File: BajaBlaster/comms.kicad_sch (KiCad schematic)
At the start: 6 parts, among them J2 Conn_01x06_Pin, J3 INTERBOARD, J4 Conn_01x04_Pin, U4 TCAN330

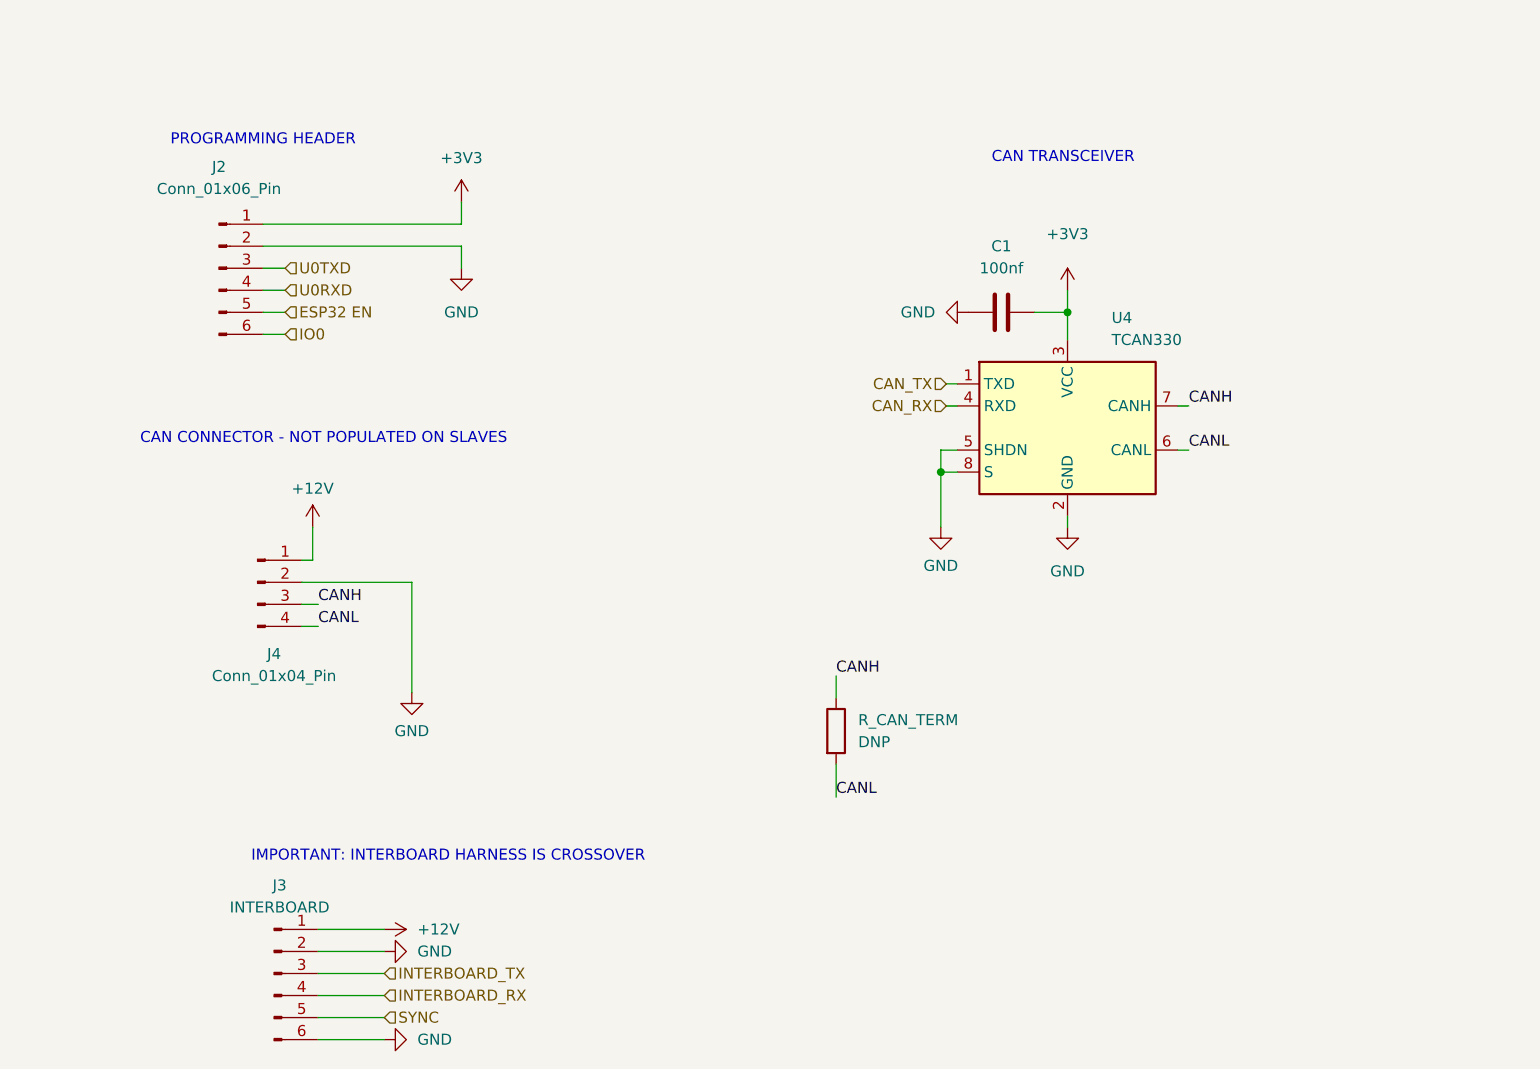
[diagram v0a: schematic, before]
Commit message: doing lots of small tweaks and fixups
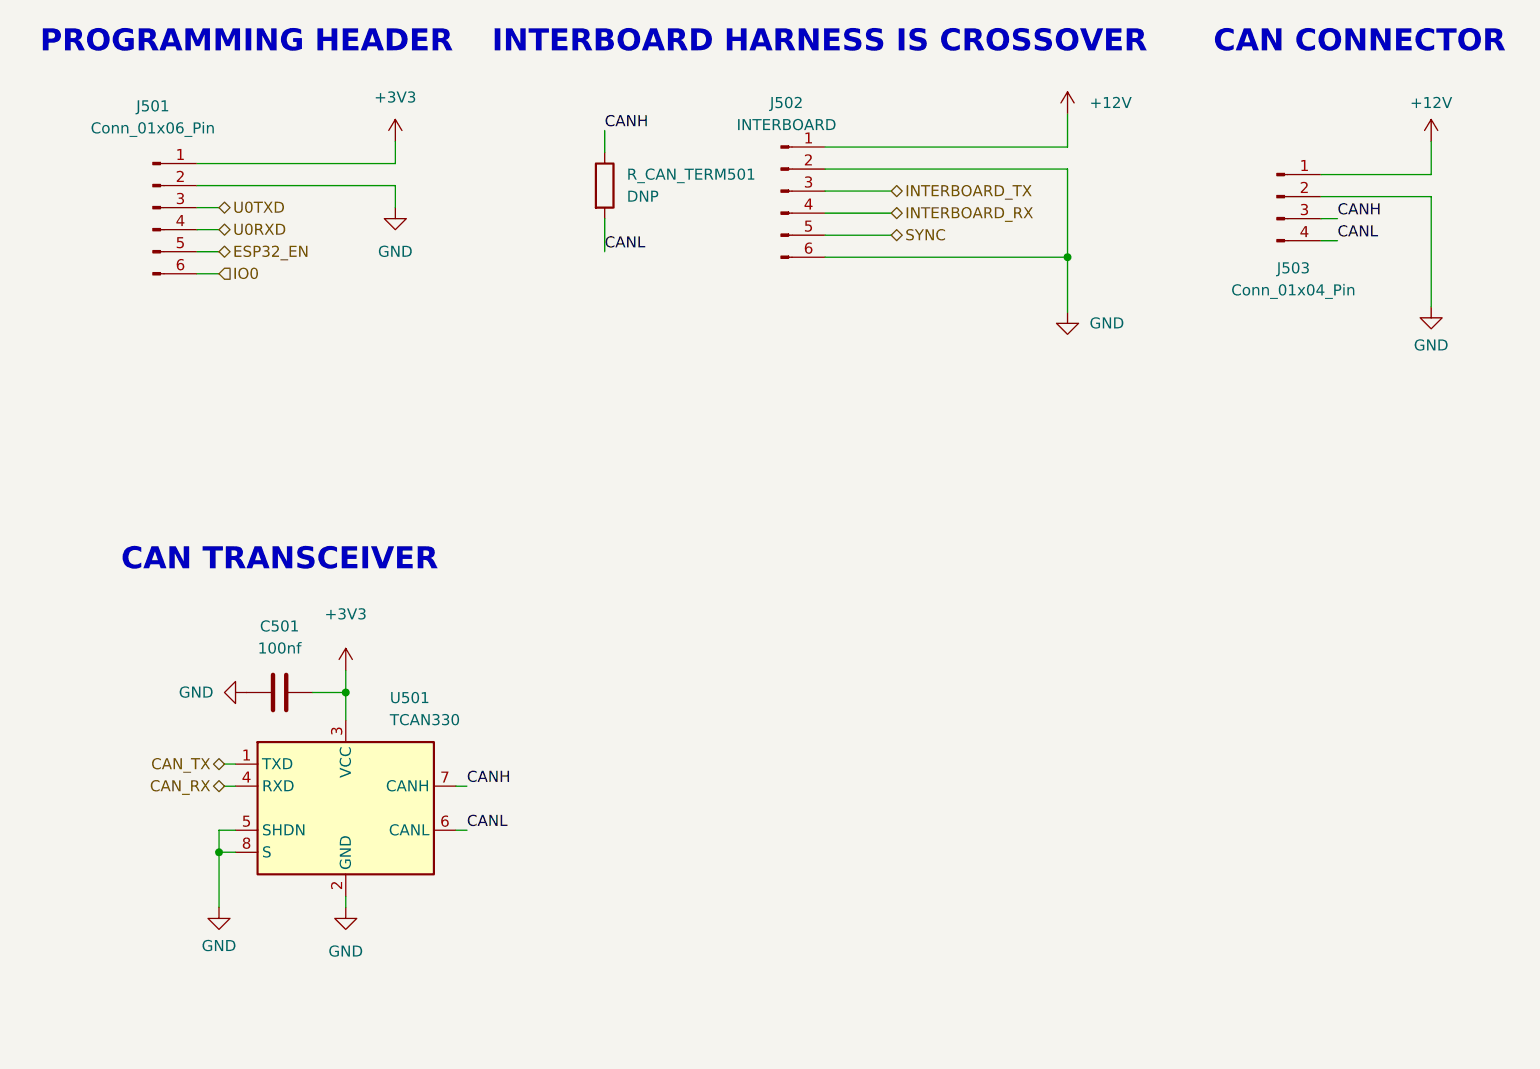
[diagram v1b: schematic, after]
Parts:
- renumbered C1 to C501, J2 to J501, J3 to J502, J4 to J503, R_CAN_TERM to R_CAN_TERM501, U4 to U501
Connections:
- net ESP32 EN renamed ESP32_EN
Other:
- note added: "CAN CONNECTOR"
- note added: "INTERBOARD HARNESS IS CROSSOVER"
- note removed: "CAN CONNECTOR - NOT POPULATED ON SLAVES"
- note removed: "IMPORTANT: INTERBOARD HARNESS IS CROSSOVER"
- title: (none) -> COMMS_REV_A
- moved on the sheet: C501, J501, J502, J503, R_CAN_TERM501, U501
